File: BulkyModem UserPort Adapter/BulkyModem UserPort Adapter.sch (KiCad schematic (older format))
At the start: 7 parts, among them J1 C64_UserPort, J2 Temporary, J3 C64_Modem_IDC, M1 Mounting, M2 Mounting, M3 Mounting, M4 Mounting

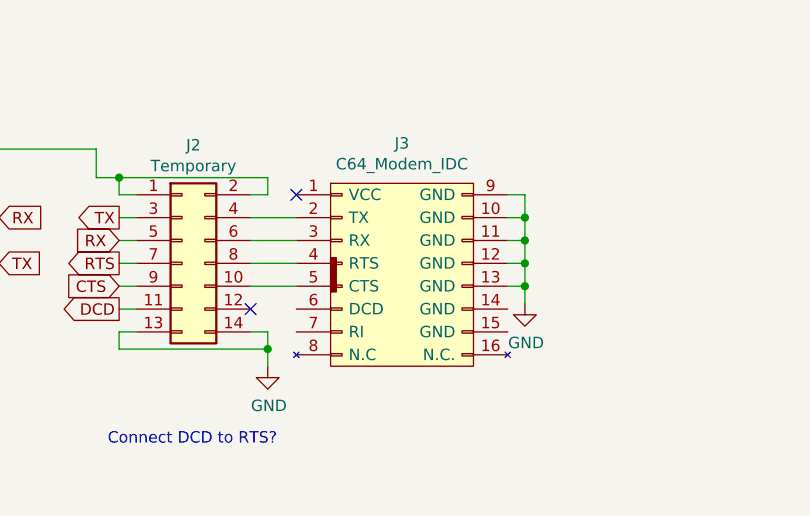
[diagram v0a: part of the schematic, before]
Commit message: Add DCD
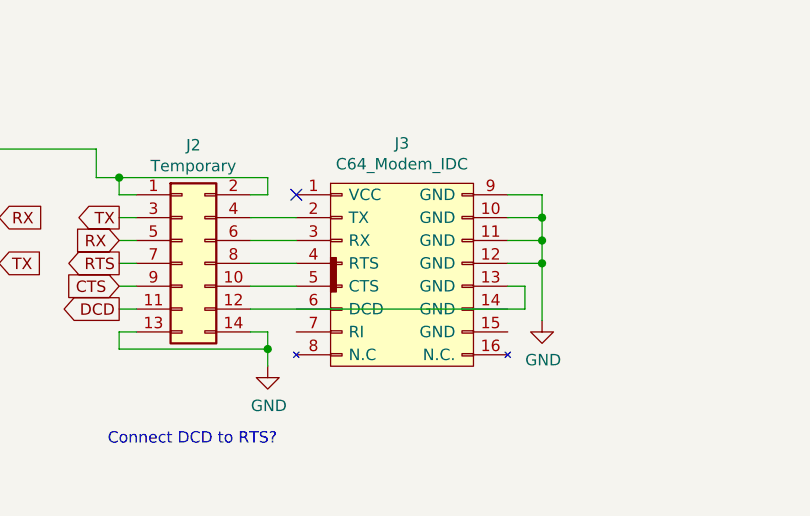
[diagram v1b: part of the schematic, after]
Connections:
- net GND: no longer J3.13 (GND)
- net at J2.12 (Pin_12): now also J3.13 (GND)
- no-connect marks 11 -> 10
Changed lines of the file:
@@
 $EndComp
 Wire Wire Line
-	8025 3575 8100 3575
+	8175 3575 8175 3675
+Connection ~ 8175 3875
+Connection ~ 8175 3775
 Wire Wire Line
-	8100 3575 8100 3675
+	8175 3775 8175 3875
+Connection ~ 8175 3675
 Wire Wire Line
-	8025 3975 8100 3975
-Connection ~ 8100 3975
-Wire Wire Line
-	8100 3975 8100 4050
-Wire Wire Line
-	8025 3875 8100 3875
-Connection ~ 8100 3875
-Wire Wire Line
-	8100 3875 8100 3975
-Wire Wire Line
-	8025 3775 8100 3775
-Connection ~ 8100 3775
-Wire Wire Line
-	8100 3775 8100 3875
-Wire Wire Line
-	8025 3675 8100 3675
-Connection ~ 8100 3675
-Wire Wire Line
-	8100 3675 8100 3775
+	8175 3675 8175 3775
 $Comp
 L power:GND #PWR0102
 U 1 1 62D9791D
-P 8100 4050
-F 0 "#PWR0102" H 8100 3800 50  0001 C CNN
-F 1 "GND" H 8105 3877 50  0000 C CNN
-F 2 "" H 8100 4050 50  0001 C CNN
-F 3 "" H 8100 4050 50  0001 C CNN
-	1    8100 4050
+P 8175 4125
+F 0 "#PWR0102" H 8175 3875 50  0001 C CNN
+F 1 "GND" H 8180 3952 50  0000 C CNN
+F 2 "" H 8175 4125 50  0001 C CNN
+F 3 "" H 8175 4125 50  0001 C CNN
+	1    8175 4125
 	1    0    0    -1
 $EndComp
@@
 NoConn ~ 5550 3575
 NoConn ~ 5550 3475
-$Comp
-L Connector_Generic:Conn_02x07_Odd_Even J2
-U 1 1 62DBC4D4
-P 6600 3875
-F 0 "J2" H 6650 4392 50  0000 C CNN
-F 1 "Temporary" H 6650 4301 50  0000 C CNN
-F 2 "Connector_PinHeader_2.54mm:PinHeader_2x07_P2.54mm_Vertical" H 6600 3875 50  0001 C CNN
-F 3 "~" H 6600 3875 50  0001 C CNN
-	1    6600 3875
-	1    0    0    -1
-$EndComp
 Wire Wire Line
 	6900 3575 6975 3575
@@
 Text GLabel 6325 4075 0    50   Output ~ 0
 DCD
-NoConn ~ 6900 4075
 Wire Wire Line
 	6325 4075 6400 4075
@@
 	6225 3500 6325 3500
 Connection ~ 6325 3500
+$Comp
+L Connector_Generic:Conn_02x07_Odd_Even J2
+U 1 1 62DBC4D4
+P 6600 3875
+F 0 "J2" H 6650 4392 50  0000 C CNN
+F 1 "Temporary" H 6650 4301 50  0000 C CNN
+F 2 "Connector_PinHeader_2.54mm:PinHeader_2x07_P2.54mm_Vertical" H 6600 3875 50  0001 C CNN
+F 3 "~" H 6600 3875 50  0001 C CNN
+	1    6600 3875
+	1    0    0    -1
+$EndComp
+Wire Wire Line
+	6900 4075 8100 4075
+Wire Wire Line
+	8100 4075 8100 3975
+Wire Wire Line
+	8100 3975 8025 3975
+Wire Wire Line
+	8025 3875 8175 3875
+Wire Wire Line
+	8025 3775 8175 3775
+Wire Wire Line
+	8025 3575 8175 3575
+Wire Wire Line
+	8025 3675 8175 3675
+Wire Wire Line
+	8175 3875 8175 4125
 $EndSCHEMATC
